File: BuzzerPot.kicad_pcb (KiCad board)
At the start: 2 copper layers, 39.1 x 24.5 mm, 12 parts, among them J1 ConnM_01x03_Horizontal_2.54mm, U1 SC8002B

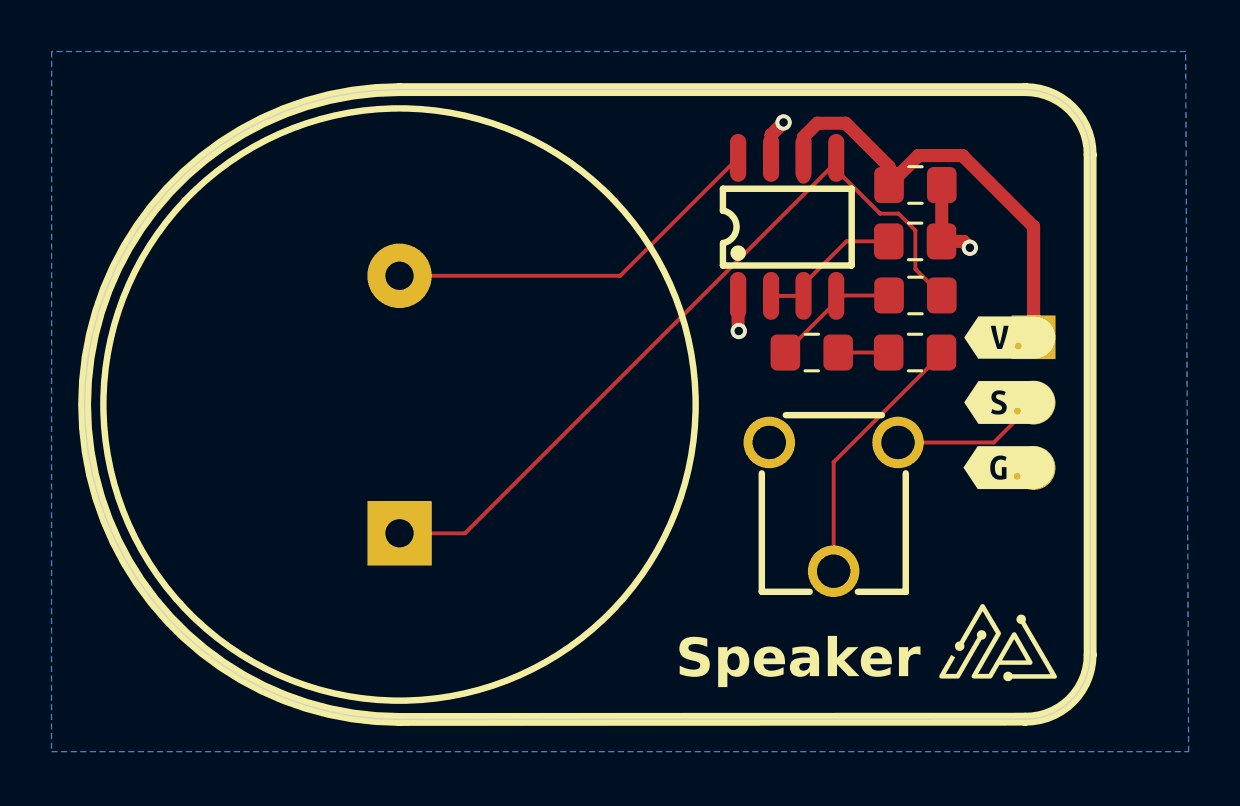
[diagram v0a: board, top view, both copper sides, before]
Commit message: Updated Version 2
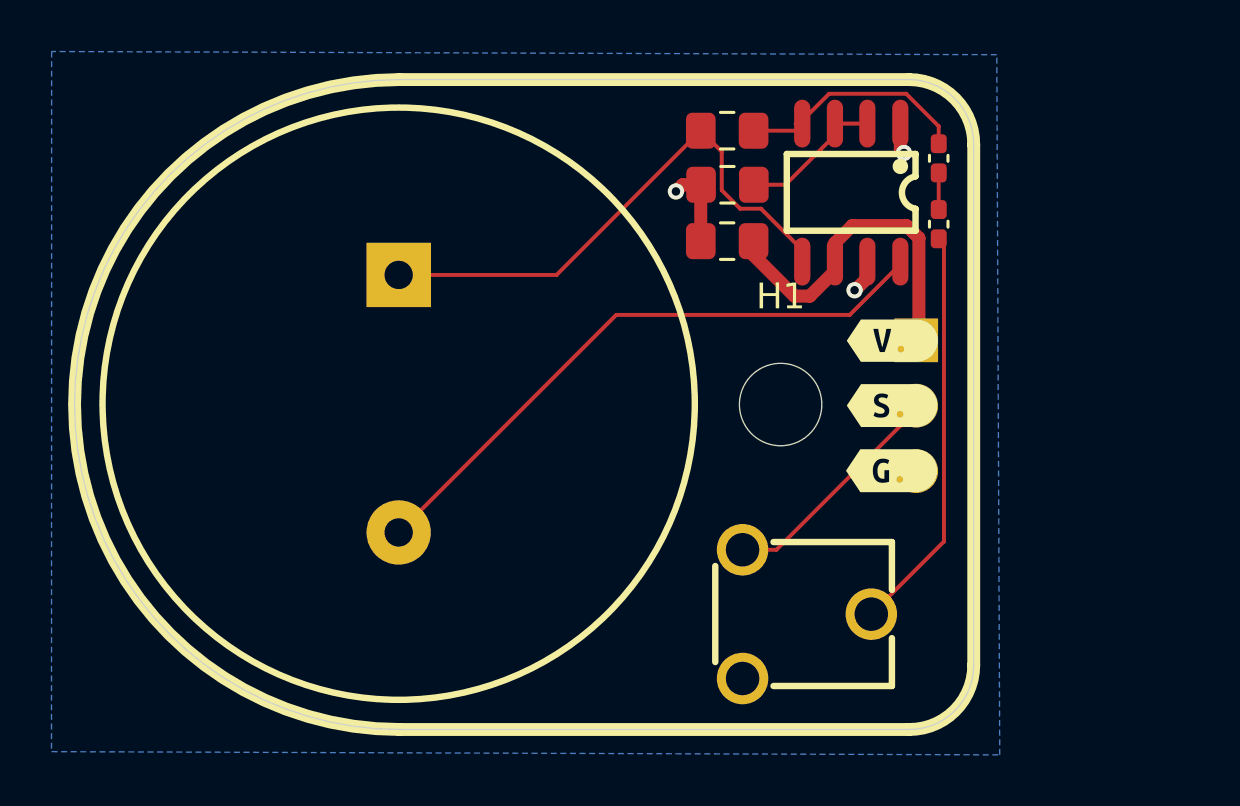
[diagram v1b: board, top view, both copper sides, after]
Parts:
- removed R1: WH06-2C-103(10K), easyeda2kicad:RES-ADJ-TH_WH06-2C-103
- added H1: MountingHole_3.2mm_M3_NoConn, Remal_KiCadLib:MountingHole_3.2mm_M3_NoConn, F.Cu at (151.2, 99.7)
- added R4: WH06-2C-103(10K), easyeda2kicad:RES-ADJ-TH_WH06-2C-103, F.Cu at (152.2, 107.9)
- C3: footprint Remal_KiCadLib:C_0805_2012m -> Remal_KiCadLib:C_0402_1005m
- R2: footprint Remal_KiCadLib:R_0805_2012m -> Remal_KiCadLib:R_0402_1005m
- moved R3 9.72 mm to (149.1, 89.1), turned to 180 degrees
- moved R2 9.01 mm to (157.3, 90.2), turned to 90 degrees
- moved C2 7.63 mm to (149.1, 93.4), turned to 180 degrees
- moved C1 7.61 mm to (149.1, 91.2), turned to 0 degrees
- moved C3 5.07 mm to (157.3, 92.7), turned to 90 degrees
- moved J1 4.56 mm to (156.4, 97.2)
- moved kibuzzard-67CEDACD 4.56 mm to (155.5, 99.8)
- moved kibuzzard-67CEDAF1 4.56 mm to (155.5, 102.3)
- moved kibuzzard-67CEDAF9 4.56 mm to (155.5, 97.2)
- moved U1 2.81 mm to (153.9, 91.5), turned to 180 degrees
- turned SPK1 to -90 degrees
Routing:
- net Net-(SPK1-+): track 30.6 -> 21.7 mm
- net Net-(SPK1--): track 15.4 -> 23.9 mm
- net Net-(C3-Pad1): track 10.2 -> 15.8 mm
- net +5V: track 19.1 -> 13.6 mm
- net Net-(U1--IN): track 5.33 -> 9.31 mm
- net SIG: track 5.91 -> 9.16 mm
- net Base: track 1.96 -> 1.42 mm
- net GND: track 6.35 -> 5.81 mm
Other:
- board size 39.1 x 24.5 mm -> 34.9 x 25.2 mm
- board text removed: "Speaker"
